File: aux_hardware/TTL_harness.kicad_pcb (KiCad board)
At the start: 2 copper layers, 34 x 67 mm, 6 parts, among them P1 CONN_01X24, P2 CONN_01X24, P3 CONN_01X02, U1 74LVC245, U2 74LVC245, U3 74LVC245

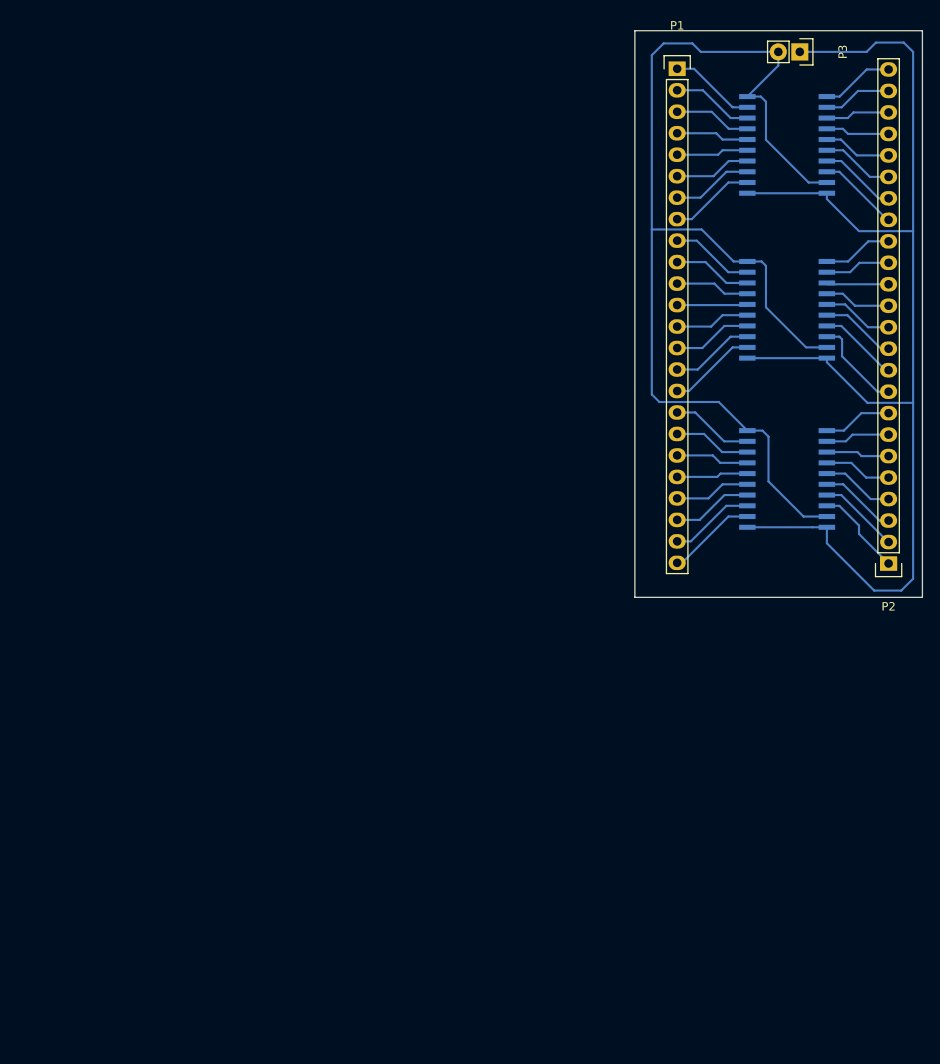
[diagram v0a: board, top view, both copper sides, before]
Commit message: Regenerated both PCBs
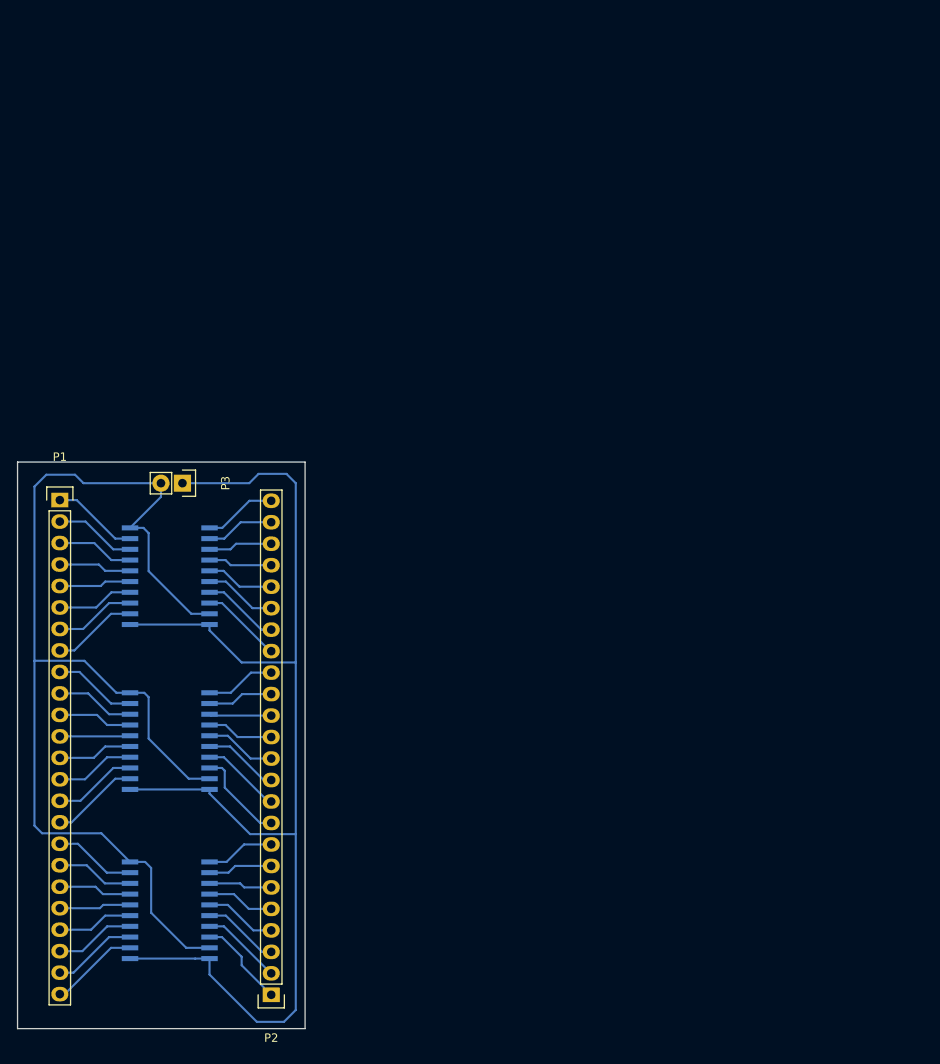
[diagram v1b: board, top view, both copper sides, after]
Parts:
- moved P1 89.1 mm to (21.0, 131.5)
- moved P2 89.1 mm to (46.0, 190.0)
- moved P3 89.1 mm to (35.5, 129.5)
- moved U1 89.1 mm to (34.0, 140.5)
- moved U2 89.1 mm to (34.0, 160.0)
- moved U3 89.1 mm to (34.0, 180.0)
